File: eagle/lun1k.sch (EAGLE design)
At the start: 103 parts, among them IC1 LTC3558, IC2 LM27313, IC3 STM32F405RGT, IC4 NRF24L01SMD, J2 XF2-3015-1LW, Q1 Q12M-SMD-S, Q2 3.2X2.5CRYSTAL, SW1 JS102011SAQN, SW2 SWITCH_MCTAEF, SW3 SWITCH_MCTAEF, SW4 SWITCH_MCTAEF, U1 N35P112, X1 MICROUSB, X1_ JST-PH3

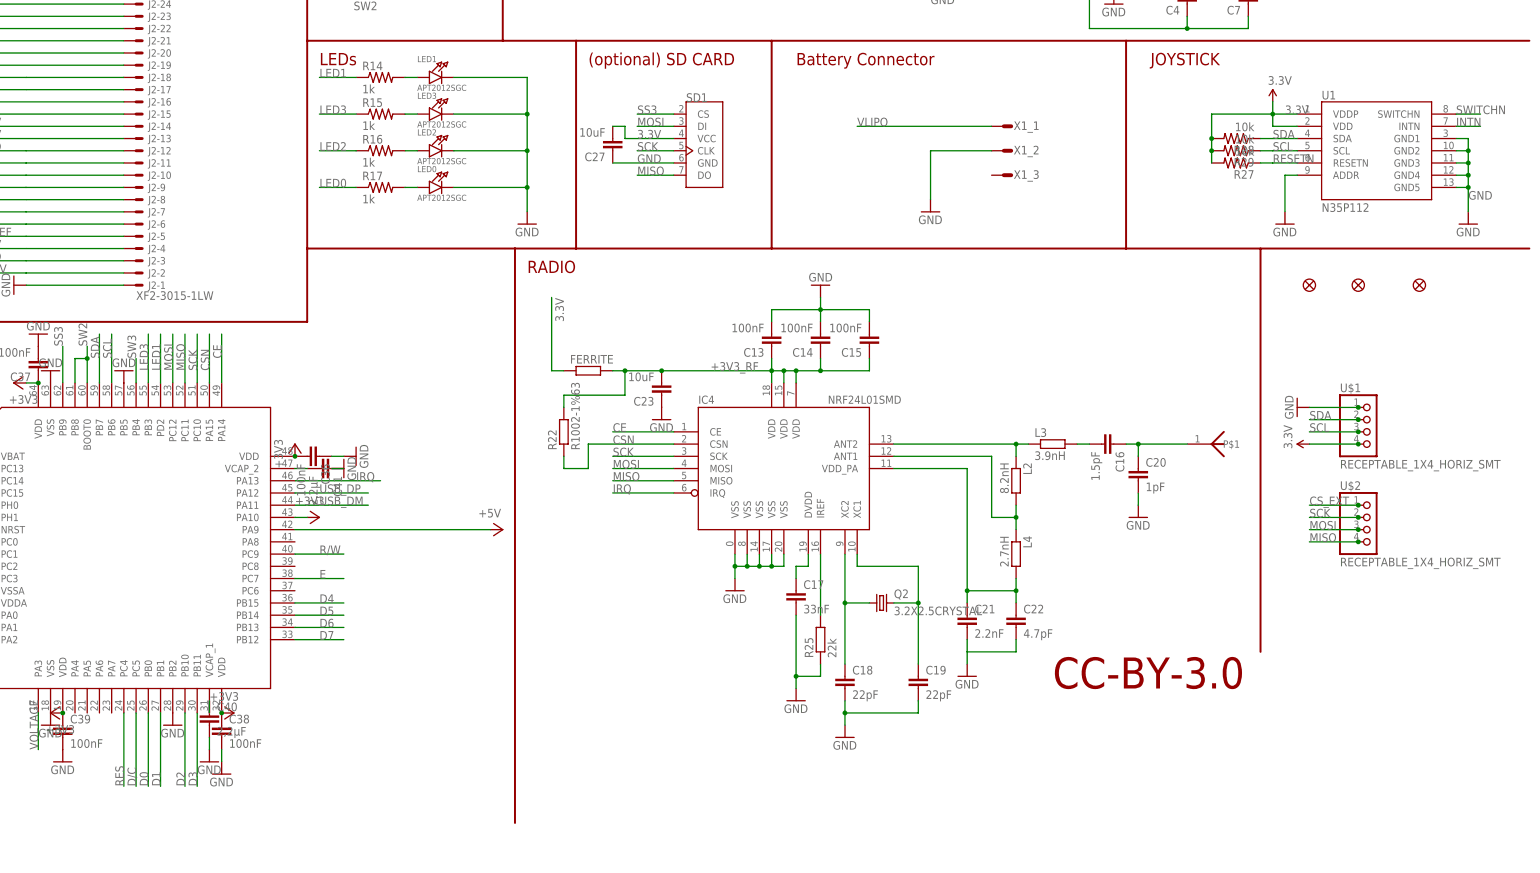
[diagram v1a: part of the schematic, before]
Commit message: routing
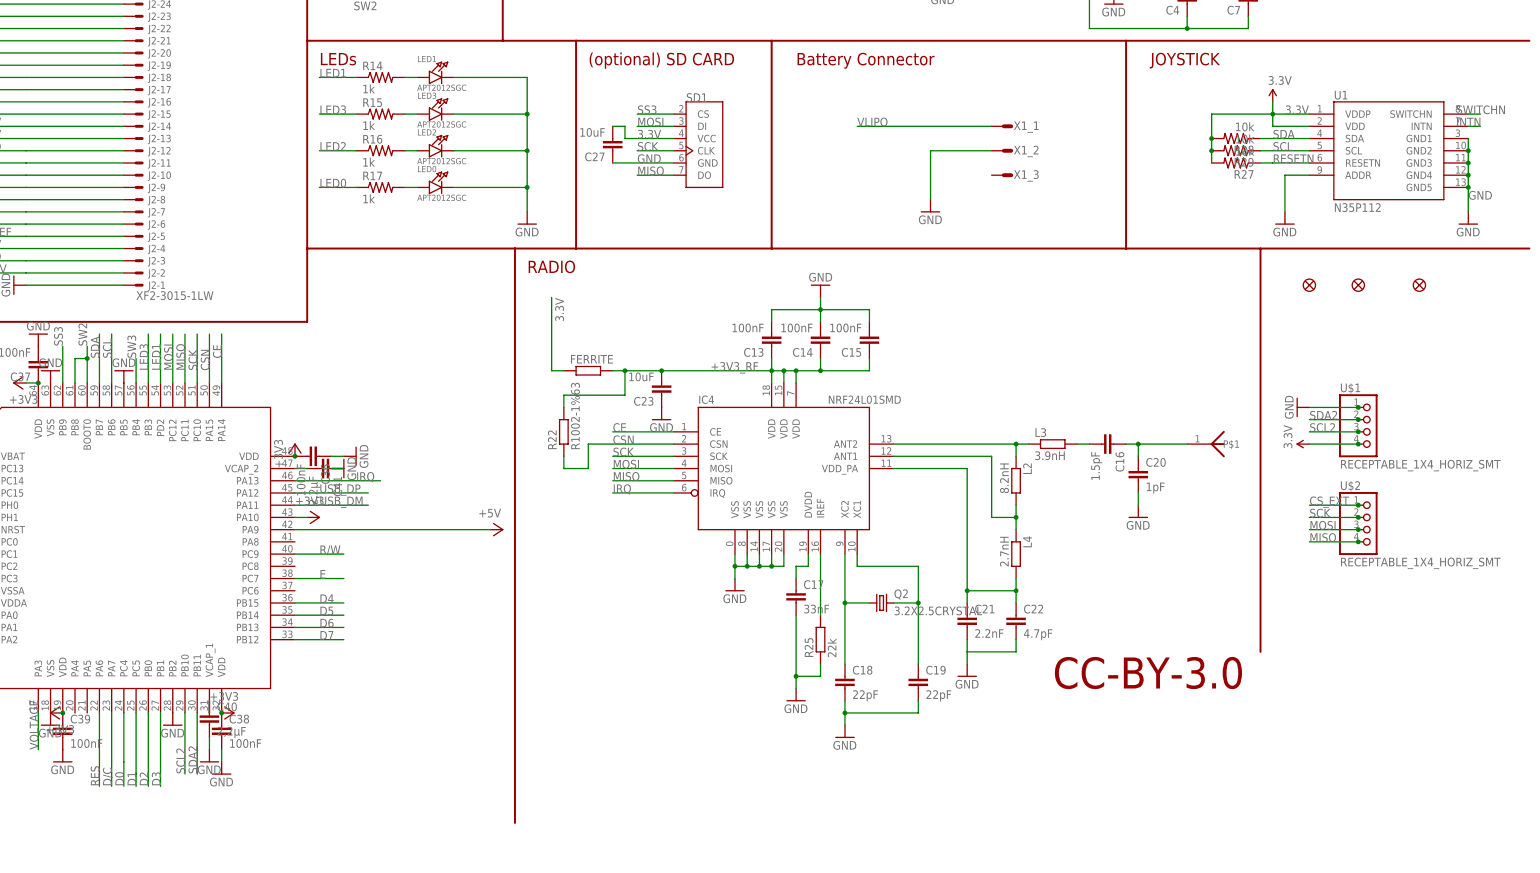
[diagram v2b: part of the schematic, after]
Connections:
- new net SCL2: IC3.PB10, U$1.3, U$1.3@1
- new net SDA2: IC3.PB11, U$1.2, U$1.2@1
- net D/C: now also IC3.PA7; no longer IC3.PC5
- net D0: now also IC3.PC4; no longer IC3.PB0
- net D1: now also IC3.PC5; no longer IC3.PB1
- net D2: now also IC3.PB0; no longer IC3.PB10
- net D3: now also IC3.PB1; no longer IC3.PB11
- net RES: now also IC3.PA6; no longer IC3.PC4
- net SCL: no longer U$1.3, U$1.3@1
- net SDA: no longer U$1.2, U$1.2@1
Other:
- moved on the sheet: U1
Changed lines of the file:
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@@
 <instance part="GND45" gate="1" x="96.52" y="93.98" rot="R180"/>
 <instance part="GND46" gate="1" x="106.68" y="20.32"/>
-<instance part="U1" gate="G$1" x="345.44" y="129.54"/>
+<instance part="U1" gate="G$1" x="347.98" y="129.54"/>
 <instance part="P+8" gate="G$1" x="335.28" y="149.86"/>
 <instance part="GND12" gate="1" x="375.92" y="124.46"/>
@@
 </segment>
 <segment>
-<wire x1="373.38" y1="142.24" x2="375.92" y2="142.24" width="0.1524" layer="91"/>
 <wire x1="375.92" y1="142.24" x2="375.92" y2="139.7" width="0.1524" layer="91"/>
 <wire x1="375.92" y1="127" x2="375.92" y2="132.08" width="0.1524" layer="91"/>
-<wire x1="373.38" y1="132.08" x2="375.92" y2="132.08" width="0.1524" layer="91"/>
 <wire x1="375.92" y1="132.08" x2="375.92" y2="134.62" width="0.1524" layer="91"/>
-<wire x1="373.38" y1="134.62" x2="375.92" y2="134.62" width="0.1524" layer="91"/>
 <wire x1="375.92" y1="134.62" x2="375.92" y2="137.16" width="0.1524" layer="91"/>
-<wire x1="373.38" y1="137.16" x2="375.92" y2="137.16" width="0.1524" layer="91"/>
 <wire x1="375.92" y1="137.16" x2="375.92" y2="139.7" width="0.1524" layer="91"/>
-<wire x1="375.92" y1="139.7" x2="373.38" y2="139.7" width="0.1524" layer="91"/>
 <junction x="375.92" y="132.08"/>
 <junction x="375.92" y="134.62"/>
@@
 <segment>
 <pinref part="U1" gate="G$1" pin="ADDR"/>
-<wire x1="340.36" y1="134.62" x2="337.82" y2="134.62" width="0.1524" layer="91"/>
+<wire x1="342.9" y1="134.62" x2="337.82" y2="134.62" width="0.1524" layer="91"/>
 <pinref part="GND1" gate="1" pin="GND"/>
 <wire x1="337.82" y1="134.62" x2="337.82" y2="127" width="0.1524" layer="91"/>
@@
 <segment>
 <wire x1="335.28" y1="149.86" x2="335.28" y2="147.32" width="0.1524" layer="91"/>
-<wire x1="335.28" y1="147.32" x2="340.36" y2="147.32" width="0.1524" layer="91"/>
-<wire x1="340.36" y1="144.78" x2="335.28" y2="144.78" width="0.1524" layer="91"/>
+<wire x1="335.28" y1="147.32" x2="342.9" y2="147.32" width="0.1524" layer="91"/>
+<wire x1="342.9" y1="144.78" x2="335.28" y2="144.78" width="0.1524" layer="91"/>
 <wire x1="335.28" y1="144.78" x2="335.28" y2="147.32" width="0.1524" layer="91"/>
 <junction x="335.28" y="147.32"/>
@@
 </segment>
 <segment>
-<pinref part="IC3" gate="G$1" pin="PC4"/>
-<wire x1="96.52" y1="22.86" x2="96.52" y2="7.62" width="0.1524" layer="91"/>
-<label x="96.52" y="7.62" size="1.778" layer="95" rot="R90"/>
+<label x="91.44" y="7.62" size="1.778" layer="95" rot="R90"/>
+<pinref part="IC3" gate="G$1" pin="PA6"/>
+<wire x1="91.44" y1="15.24" x2="91.44" y2="7.62" width="0.1524" layer="91"/>
+<wire x1="91.44" y1="15.24" x2="91.44" y2="22.86" width="0.1524" layer="91"/>
 </segment>
 </net>
@@
 </segment>
 <segment>
-<pinref part="IC3" gate="G$1" pin="PC5"/>
-<wire x1="99.06" y1="22.86" x2="99.06" y2="7.62" width="0.1524" layer="91"/>
-<label x="99.06" y="7.62" size="1.778" layer="95" rot="R90"/>
+<label x="93.98" y="7.62" size="1.778" layer="95" rot="R90"/>
+<pinref part="IC3" gate="G$1" pin="PA7"/>
+<wire x1="93.98" y1="12.7" x2="93.98" y2="7.62" width="0.1524" layer="91"/>
+<wire x1="93.98" y1="12.7" x2="93.98" y2="22.86" width="0.1524" layer="91"/>
 </segment>
 </net>
@@
 </segment>
 <segment>
-<pinref part="IC3" gate="G$1" pin="PB1"/>
-<wire x1="104.14" y1="22.86" x2="104.14" y2="7.62" width="0.1524" layer="91"/>
-<label x="104.14" y="7.62" size="1.778" layer="95" rot="R90"/>
+<label x="99.06" y="7.62" size="1.778" layer="95" rot="R90"/>
+<pinref part="IC3" gate="G$1" pin="PC5"/>
+<wire x1="99.06" y1="10.16" x2="99.06" y2="7.62" width="0.1524" layer="91"/>
+<wire x1="99.06" y1="10.16" x2="99.06" y2="22.86" width="0.1524" layer="91"/>
 </segment>
 </net>
@@
 </segment>
 <segment>
-<pinref part="IC3" gate="G$1" pin="PB0"/>
-<wire x1="101.6" y1="22.86" x2="101.6" y2="7.62" width="0.1524" layer="91"/>
-<label x="101.6" y="7.62" size="1.778" layer="95" rot="R90"/>
+<label x="96.52" y="7.62" size="1.778" layer="95" rot="R90"/>
+<pinref part="IC3" gate="G$1" pin="PC4"/>
+<wire x1="96.52" y1="12.7" x2="96.52" y2="7.62" width="0.1524" layer="91"/>
+<wire x1="96.52" y1="12.7" x2="96.52" y2="22.86" width="0.1524" layer="91"/>
 </segment>
 </net>
@@
 <net name="SDA" class="0">
 <segment>
-<wire x1="335.28" y1="142.24" x2="340.36" y2="142.24" width="0.1524" layer="91"/>
+<wire x1="332.74" y1="142.24" x2="342.9" y2="142.24" width="0.1524" layer="91"/>
 <label x="335.28" y="142.24" size="1.778" layer="95"/>
 <pinref part="U1" gate="G$1" pin="SDA"/>
-</segment>
-<segment>
-<wire x1="332.74" y1="142.24" x2="335.28" y2="142.24" width="0.1524" layer="91"/>
 <pinref part="R28" gate="G$1" pin="1"/>
-<wire x1="342.9" y1="83.82" x2="353.06" y2="83.82" width="0.1524" layer="91"/>
-<pinref part="U$1" gate="G$1" pin="2"/>
-<pinref part="U$1" gate="G$1" pin="2@1"/>
-<junction x="353.06" y="83.82"/>
-<label x="342.9" y="83.82" size="1.778" layer="95"/>
 </segment>
 <segment>
@@
 <net name="SCL" class="0">
 <segment>
-<wire x1="335.28" y1="139.7" x2="340.36" y2="139.7" width="0.1524" layer="91"/>
-<label x="335.28" y="139.7" size="1.778" layer="95"/>
-<pinref part="U1" gate="G$1" pin="SCL"/>
-<wire x1="342.9" y1="81.28" x2="353.06" y2="81.28" width="0.1524" layer="91"/>
-<pinref part="U$1" gate="G$1" pin="3"/>
-<pinref part="U$1" gate="G$1" pin="3@1"/>
-<junction x="353.06" y="81.28"/>
-<label x="342.9" y="81.28" size="1.778" layer="95"/>
-</segment>
-<segment>
-<wire x1="332.74" y1="139.7" x2="335.28" y2="139.7" width="0.1524" layer="91"/>
-<pinref part="R29" gate="G$1" pin="1"/>
-</segment>
-<segment>
 <pinref part="IC3" gate="G$1" pin="PB6"/>
 <wire x1="93.98" y1="91.44" x2="93.98" y2="101.6" width="0.1524" layer="91"/>
 <label x="93.98" y="96.52" size="1.778" layer="95" rot="R90"/>
 </segment>
+<segment>
+<wire x1="332.74" y1="139.7" x2="342.9" y2="139.7" width="0.1524" layer="91"/>
+<pinref part="U1" gate="G$1" pin="SCL"/>
+<pinref part="R29" gate="G$1" pin="1"/>
+<label x="335.28" y="139.7" size="1.778" layer="95"/>
+</segment>
 </net>
 <net name="RESETN" class="0">
 <segment>
-<wire x1="340.36" y1="137.16" x2="335.28" y2="137.16" width="0.1524" layer="91"/>
+<wire x1="342.9" y1="137.16" x2="335.28" y2="137.16" width="0.1524" layer="91"/>
 <label x="335.28" y="137.16" size="1.778" layer="95"/>
 <pinref part="U1" gate="G$1" pin="RESETN"/>
@@
 <net name="INTN" class="0">
 <segment>
-<wire x1="373.38" y1="144.78" x2="378.46" y2="144.78" width="0.1524" layer="91"/>
+<wire x1="375.92" y1="144.78" x2="378.46" y2="144.78" width="0.1524" layer="91"/>
 <label x="373.38" y="144.78" size="1.778" layer="95"/>
 <pinref part="U1" gate="G$1" pin="INTN"/>
@@
 <net name="SWITCHN" class="0">
 <segment>
-<wire x1="373.38" y1="147.32" x2="378.46" y2="147.32" width="0.1524" layer="91"/>
+<wire x1="375.92" y1="147.32" x2="378.46" y2="147.32" width="0.1524" layer="91"/>
 <label x="373.38" y="147.32" size="1.778" layer="95"/>
 <pinref part="U1" gate="G$1" pin="SWITCHN"/>
@@
 </segment>
 <segment>
-<pinref part="IC3" gate="G$1" pin="PB10"/>
-<wire x1="109.22" y1="22.86" x2="109.22" y2="7.62" width="0.1524" layer="91"/>
-<label x="109.22" y="7.62" size="1.778" layer="95" rot="R90"/>
+<label x="101.6" y="7.62" size="1.778" layer="95" rot="R90"/>
+<pinref part="IC3" gate="G$1" pin="PB0"/>
+<wire x1="101.6" y1="10.16" x2="101.6" y2="7.62" width="0.1524" layer="91"/>
+<wire x1="101.6" y1="10.16" x2="101.6" y2="22.86" width="0.1524" layer="91"/>
 </segment>
 </net>
@@
 </segment>
 <segment>
-<pinref part="IC3" gate="G$1" pin="PB11"/>
-<wire x1="111.76" y1="22.86" x2="111.76" y2="7.62" width="0.1524" layer="91"/>
-<label x="111.76" y="7.62" size="1.778" layer="95" rot="R90"/>
+<label x="104.14" y="7.62" size="1.778" layer="95" rot="R90"/>
+<pinref part="IC3" gate="G$1" pin="PB1"/>
+<wire x1="104.14" y1="12.7" x2="104.14" y2="7.62" width="0.1524" layer="91"/>
+<wire x1="104.14" y1="12.7" x2="104.14" y2="22.86" width="0.1524" layer="91"/>
 </segment>
 </net>
@@
 </segment>
 </net>
+<net name="SDA2" class="0">
+<segment>
+<pinref part="IC3" gate="G$1" pin="PB11"/>
+<wire x1="111.76" y1="22.86" x2="111.76" y2="10.16" width="0.1524" layer="91"/>
+<label x="111.76" y="10.16" size="1.778" layer="95" rot="R90"/>
+</segment>
+<segment>
+<wire x1="342.9" y1="83.82" x2="353.06" y2="83.82" width="0.1524" layer="91"/>
+<pinref part="U$1" gate="G$1" pin="2"/>
+<pinref part="U$1" gate="G$1" pin="2@1"/>
+<junction x="353.06" y="83.82"/>
+<label x="342.9" y="83.82" size="1.778" layer="95"/>
+</segment>
+</net>
+<net name="SCL2" class="0">
+<segment>
+<pinref part="IC3" gate="G$1" pin="PB10"/>
+<wire x1="109.22" y1="22.86" x2="109.22" y2="10.16" width="0.1524" layer="91"/>
+<label x="109.22" y="10.16" size="1.778" layer="95" rot="R90"/>
+</segment>
+<segment>
+<pinref part="U$1" gate="G$1" pin="3"/>
+<pinref part="U$1" gate="G$1" pin="3@1"/>
+<wire x1="353.06" y1="81.28" x2="342.9" y2="81.28" width="0.1524" layer="91"/>
+<junction x="353.06" y="81.28"/>
+<label x="342.9" y="81.28" size="1.778" layer="95"/>
+</segment>
+</net>

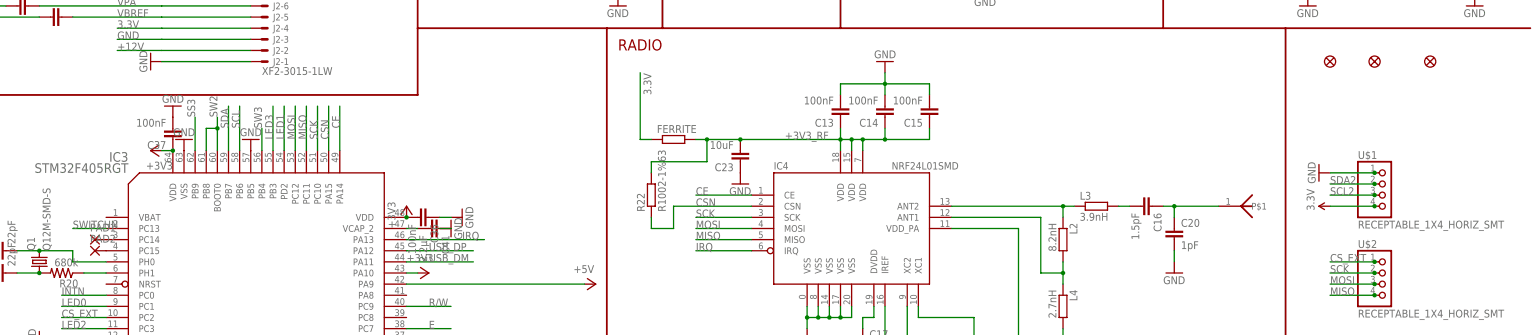
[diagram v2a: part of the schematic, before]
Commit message: routing
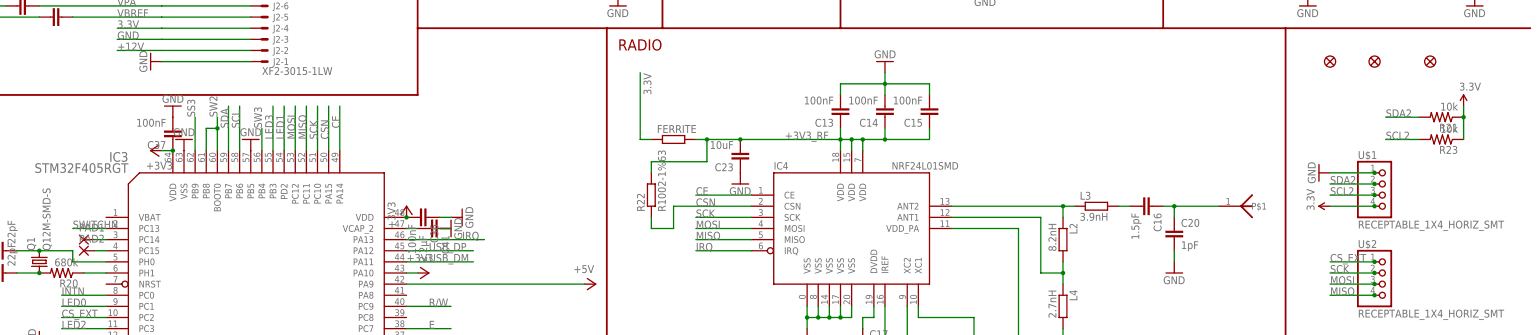
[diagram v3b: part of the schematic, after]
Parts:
- added R21, R23: 10k, SparkFun:RESISTOR0402-RES
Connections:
- net 3.3V: now also R21.1, R23.1
- net SCL2: now also R23.2
- net SDA2: now also R21.2
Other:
- moved on the sheet: PAD1, PAD2
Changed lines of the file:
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@@
 <part name="R20" library="SparkFun-Resistors" deviceset="RESISTOR" device="0402-RES" value="680k"/>
 <part name="U$2" library="seb" deviceset="RECEPTABLE_1X4_HORIZ_SMT" device=""/>
+<part name="R21" library="SparkFun" deviceset="RESISTOR" device="0402-RES" value="10k"/>
+<part name="R23" library="SparkFun" deviceset="RESISTOR" device="0402-RES" value="10k"/>
+<part name="P+4" library="SparkFun" deviceset="3.3V" device=""/>
 </parts>
 <sheets>
@@
 <instance part="GND32" gate="1" x="340.36" y="86.36" rot="R270"/>
 <instance part="P+3" gate="G$1" x="342.9" y="78.74" rot="R90"/>
-<instance part="PAD1" gate="1" x="60.96" y="71.12"/>
-<instance part="PAD2" gate="1" x="60.96" y="68.58"/>
+<instance part="PAD1" gate="1" x="58.42" y="71.12"/>
+<instance part="PAD2" gate="1" x="58.42" y="68.58"/>
 <instance part="D1" gate="G$1" x="233.68" y="-25.4"/>
 <instance part="L5" gate="G$1" x="210.82" y="-25.4" rot="R90"/>
@@
 <instance part="R20" gate="G$1" x="53.34" y="63.5" rot="R180"/>
 <instance part="U$2" gate="G$1" x="353.06" y="60.96"/>
+<instance part="R21" gate="G$1" x="368.3" y="99.06" rot="R180"/>
+<instance part="R23" gate="G$1" x="368.3" y="93.98" rot="R180"/>
+<instance part="P+4" gate="G$1" x="373.38" y="101.6"/>
 </instances>
 <busses>
@@
 <pinref part="C33" gate="G$1" pin="1"/>
 <pinref part="R11" gate="G$1" pin="2"/>
+</segment>
+<segment>
+<pinref part="R23" gate="G$1" pin="1"/>
+<pinref part="R21" gate="G$1" pin="1"/>
+<wire x1="373.38" y1="93.98" x2="373.38" y2="99.06" width="0.1524" layer="91"/>
+<wire x1="373.38" y1="99.06" x2="373.38" y2="101.6" width="0.1524" layer="91"/>
+<junction x="373.38" y="99.06"/>
+<pinref part="P+4" gate="G$1" pin="3.3V"/>
 </segment>
 </net>
@@
 <pinref part="IC3" gate="G$1" pin="PC14"/>
 <pinref part="PAD1" gate="1" pin="P"/>
+<wire x1="60.96" y1="71.12" x2="63.5" y2="71.12" width="0.1524" layer="91"/>
 </segment>
 </net>
@@
 <pinref part="IC3" gate="G$1" pin="PC15"/>
 <pinref part="PAD2" gate="1" pin="P"/>
+<wire x1="60.96" y1="68.58" x2="63.5" y2="68.58" width="0.1524" layer="91"/>
 </segment>
 </net>
@@
 <label x="342.9" y="83.82" size="1.778" layer="95"/>
 </segment>
+<segment>
+<pinref part="R21" gate="G$1" pin="2"/>
+<wire x1="363.22" y1="99.06" x2="355.6" y2="99.06" width="0.1524" layer="91"/>
+<label x="355.6" y="99.06" size="1.778" layer="95"/>
+</segment>
 </net>
 <net name="SCL2" class="0">
@@
 <label x="342.9" y="81.28" size="1.778" layer="95"/>
 </segment>
-</net>
+<segment>
+<pinref part="R23" gate="G$1" pin="2"/>
+<wire x1="363.22" y1="93.98" x2="355.6" y2="93.98" width="0.1524" layer="91"/>
+<label x="355.6" y="93.98" size="1.778" layer="95"/>
+</segment>
+</net>
